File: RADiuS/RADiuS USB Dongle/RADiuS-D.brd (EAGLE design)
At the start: 20.3 x 57.2 mm, 13 parts

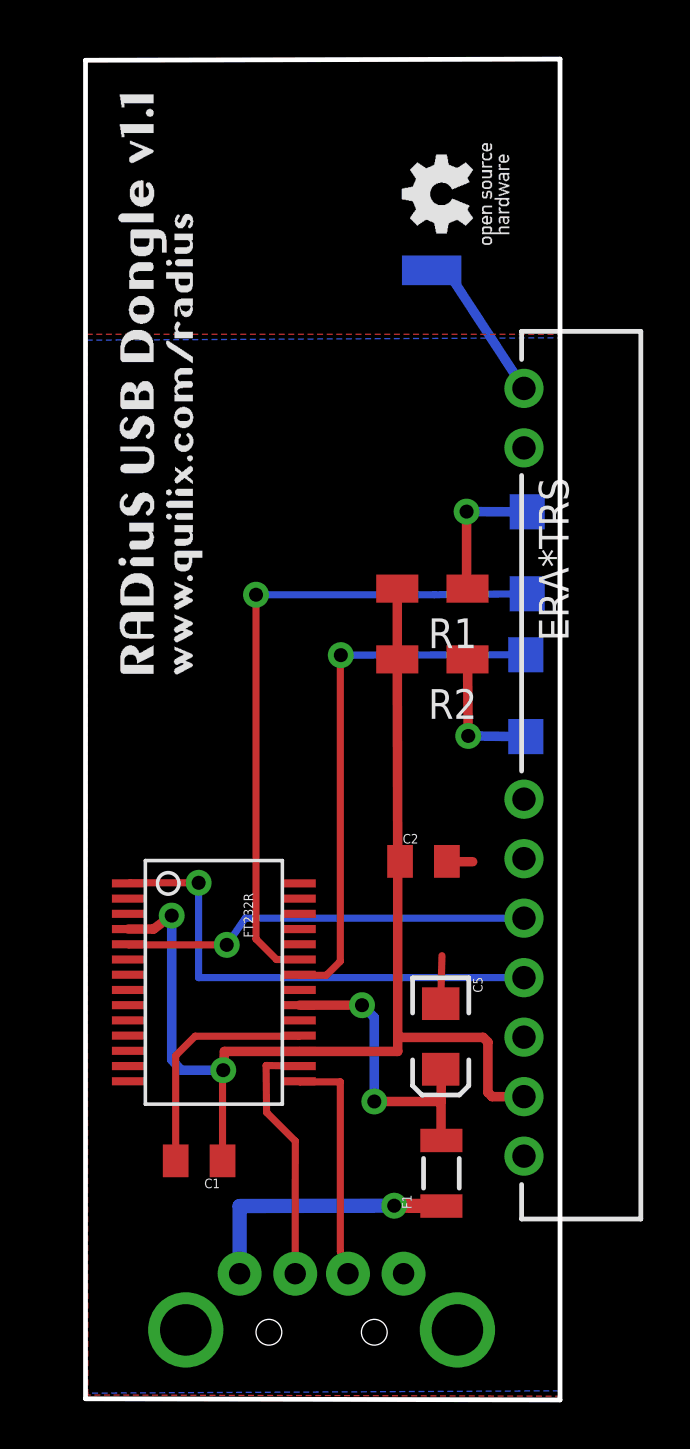
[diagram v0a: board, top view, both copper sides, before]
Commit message: production update for RADiuS projects
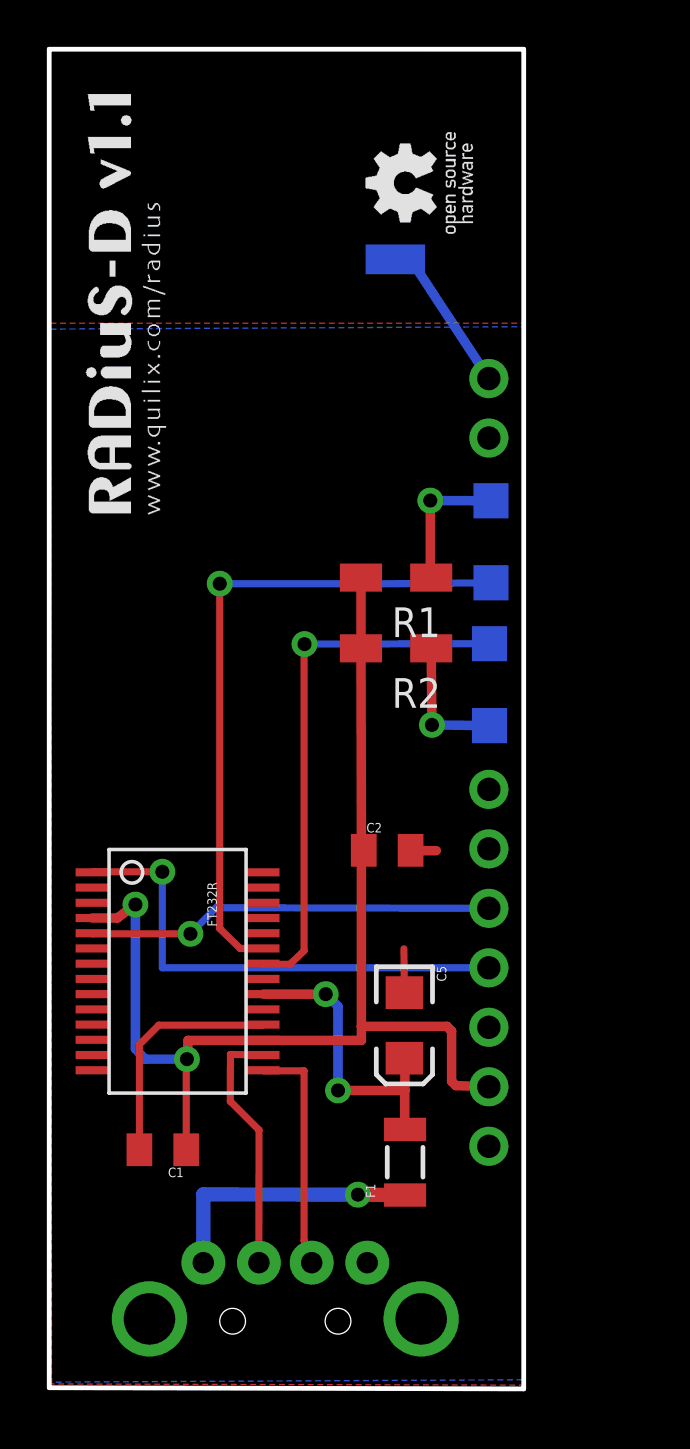
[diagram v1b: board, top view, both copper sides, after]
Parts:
- removed U$1: CREATIVE_COMMONS, SparkFun:CREATIVE_COMMONS
- moved ERA*TRS 3.61 mm to (22.0, 27.6), flipped to the bottom
- moved R1 1.62 mm to (15.5, 35.6)
- moved R2 1.62 mm to (15.5, 32.5)
- moved C2 1.62 mm to (15.1, 23.9)
- moved C5 1.62 mm to (15.9, 16.4)
- moved ANT 1.62 mm to (15.5, 49.2)
- moved C1 1.62 mm to (5.54, 11.1)
- moved FT232R 1.62 mm to (6.17, 18.8)
- moved LED1 1.62 mm to (19.5, 37.1)
- moved USB 1.62 mm to (10.8, 3.92)
- moved F1 1.62 mm to (15.9, 10.6)
- moved LED2 1.62 mm to (19.5, 31.0)
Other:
- outline, holes or cut-outs redrawn
